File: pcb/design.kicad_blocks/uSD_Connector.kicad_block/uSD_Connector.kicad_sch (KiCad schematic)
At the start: 10 parts, among them J3 0472192001

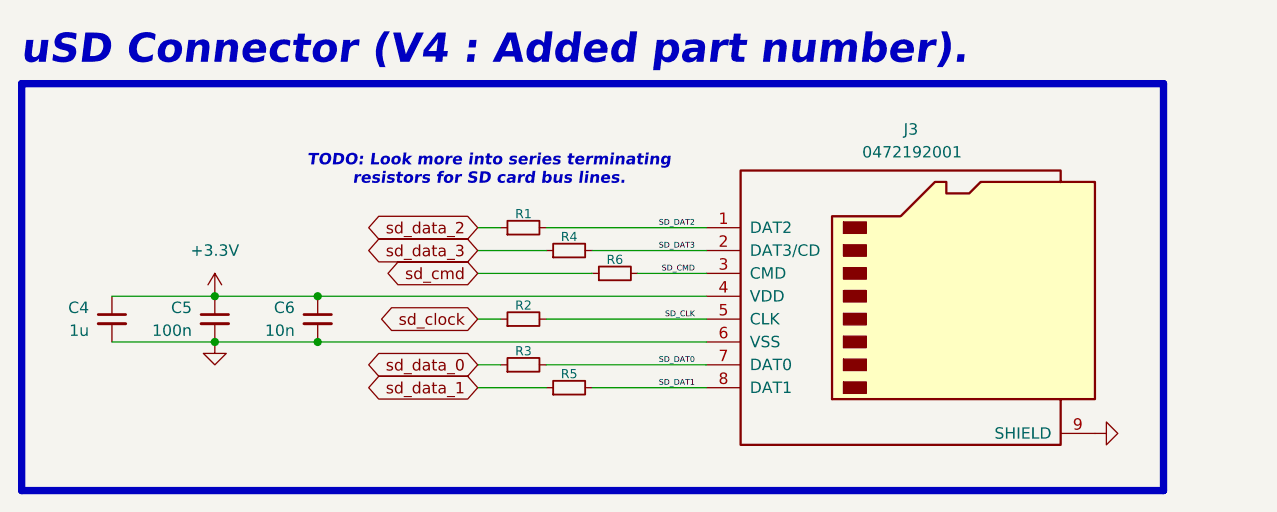
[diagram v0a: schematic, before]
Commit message: Addressed ERC issues.
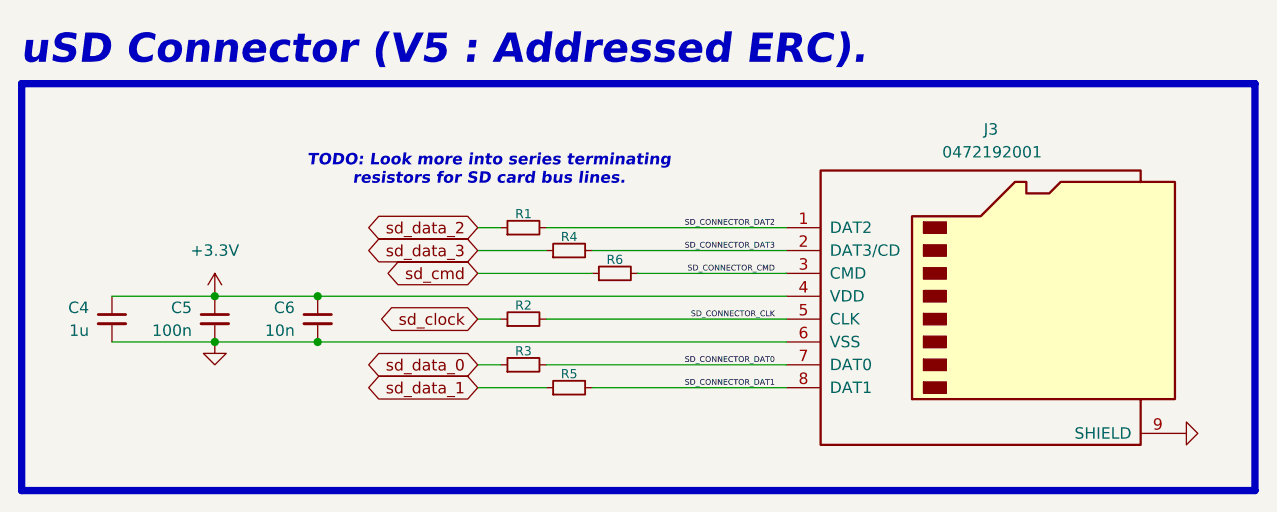
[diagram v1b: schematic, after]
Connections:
- net SD_CLK renamed SD_CONNECTOR_CLK
- net SD_CMD renamed SD_CONNECTOR_CMD
- net SD_DAT0 renamed SD_CONNECTOR_DAT0
- net SD_DAT1 renamed SD_CONNECTOR_DAT1
- net SD_DAT2 renamed SD_CONNECTOR_DAT2
- net SD_DAT3 renamed SD_CONNECTOR_DAT3
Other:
- note added: "uSD Connector (V5 : Addressed ERC)."
- note removed: "uSD Connector (V4 : Added part number)."
- moved on the sheet: J3
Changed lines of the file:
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@@
 	(rectangle
 		(start 340.487 166.878)
-		(end 467.36 212.09)
+		(end 477.52 212.09)
 		(stroke
 			(width 0.8128)
@@
 		)
 	)
-	(text "uSD Connector (V4 : Added part number)."
+	(text "uSD Connector (V5 : Addressed ERC)."
 		(exclude_from_sim no)
 		(at 340.36 165.1 0)
@@
 	(wire
 		(pts
-			(xy 398.78 182.88) (xy 416.56 182.88)
-		)
-		(stroke
-			(width 0)
-			(type default)
-		)
-	)
-	(wire
-		(pts
-			(xy 403.86 200.66) (xy 416.56 200.66)
-		)
-		(stroke
-			(width 0)
-			(type default)
-		)
-	)
-	(wire
-		(pts
-			(xy 373.38 195.58) (xy 416.56 195.58)
-		)
-		(stroke
-			(width 0)
-			(type default)
-		)
-	)
-	(wire
-		(pts
 			(xy 361.95 195.58) (xy 350.52 195.58)
 		)
@@
 	(wire
 		(pts
-			(xy 403.86 185.42) (xy 416.56 185.42)
-		)
-		(stroke
-			(width 0)
-			(type default)
-		)
-	)
-	(wire
-		(pts
-			(xy 398.78 198.12) (xy 416.56 198.12)
+			(xy 373.38 190.5) (xy 425.45 190.5)
+		)
+		(stroke
+			(width 0)
+			(type default)
+		)
+	)
+	(wire
+		(pts
+			(xy 403.86 185.42) (xy 425.45 185.42)
 		)
 		(stroke
@@
 	(wire
 		(pts
+			(xy 408.94 187.96) (xy 425.45 187.96)
+		)
+		(stroke
+			(width 0)
+			(type default)
+		)
+	)
+	(wire
+		(pts
 			(xy 361.95 190.5) (xy 373.38 190.5)
 		)
@@
 	(wire
 		(pts
+			(xy 398.78 193.04) (xy 425.45 193.04)
+		)
+		(stroke
+			(width 0)
+			(type default)
+		)
+	)
+	(wire
+		(pts
+			(xy 403.86 200.66) (xy 425.45 200.66)
+		)
+		(stroke
+			(width 0)
+			(type default)
+		)
+	)
+	(wire
+		(pts
 			(xy 393.7 182.88) (xy 391.16 182.88)
 		)
@@
 	(wire
 		(pts
+			(xy 398.78 198.12) (xy 425.45 198.12)
+		)
+		(stroke
+			(width 0)
+			(type default)
+		)
+	)
+	(wire
+		(pts
+			(xy 373.38 195.58) (xy 425.45 195.58)
+		)
+		(stroke
+			(width 0)
+			(type default)
+		)
+	)
+	(wire
+		(pts
 			(xy 350.52 190.5) (xy 361.95 190.5)
 		)
@@
 	(wire
 		(pts
-			(xy 373.38 190.5) (xy 416.56 190.5)
-		)
-		(stroke
-			(width 0)
-			(type default)
-		)
-	)
-	(wire
-		(pts
-			(xy 398.78 193.04) (xy 416.56 193.04)
+			(xy 398.78 182.88) (xy 425.45 182.88)
 		)
 		(stroke
@@
 		)
 	)
-	(wire
-		(pts
-			(xy 408.94 187.96) (xy 416.56 187.96)
-		)
-		(stroke
-			(width 0)
-			(type default)
-		)
-	)
-	(label "SD_CMD"
-		(at 415.29 187.96 180)
+	(label "SD_CONNECTOR_CMD"
+		(at 424.18 187.96 180)
 		(effects
 			(font
@@
 		)
 	)
-	(label "SD_CLK"
-		(at 415.29 193.04 180)
+	(label "SD_CONNECTOR_CLK"
+		(at 424.18 193.04 180)
 		(effects
 			(font
@@
 		)
 	)
-	(label "SD_DAT0"
-		(at 415.29 198.12 180)
+	(label "SD_CONNECTOR_DAT0"
+		(at 424.18 198.12 180)
 		(effects
 			(font
@@
 		)
 	)
-	(label "SD_DAT3"
-		(at 415.29 185.42 180)
+	(label "SD_CONNECTOR_DAT3"
+		(at 424.18 185.42 180)
 		(effects
 			(font
@@
 		)
 	)
-	(label "SD_DAT2"
-		(at 415.29 182.88 180)
+	(label "SD_CONNECTOR_DAT2"
+		(at 424.18 182.88 180)
 		(effects
 			(font
@@
 		)
 	)
-	(label "SD_DAT1"
-		(at 415.29 200.66 180)
+	(label "SD_CONNECTOR_DAT1"
+		(at 424.18 200.66 180)
 		(effects
 			(font
@@
 	(symbol
 		(lib_id "Connector:Micro_SD_Card")
-		(at 439.42 190.5 0)
+		(at 448.31 190.5 0)
 		(unit 1)
 		(exclude_from_sim no)
@@
 		(dnp no)
 		(property "Reference" "J3"
-			(at 439.293 171.958 0)
+			(at 448.183 171.958 0)
 			(effects
 				(font
@@
 		)
 		(property "Value" "0472192001"
-			(at 439.42 174.498 0)
+			(at 448.31 174.498 0)
 			(effects
 				(font
@@
 		)
 		(property "Footprint" "pcb:microSD_HC_Molex_47219-2001"
-			(at 468.63 182.88 0)
+			(at 477.52 182.88 0)
 			(effects
 				(font
@@
 		)
 		(property "Datasheet" "https://www.we-online.com/components/products/datasheet/693072010801.pdf"
-			(at 439.42 190.5 0)
+			(at 448.31 190.5 0)
 			(effects
 				(font
@@
 		)
 		(property "Description" "Micro SD Card Socket"
-			(at 439.42 190.5 0)
+			(at 448.31 190.5 0)
 			(effects
 				(font
@@
 	(symbol
 		(lib_id "power:GND")
-		(at 459.74 205.74 90)
+		(at 468.63 205.74 90)
 		(unit 1)
 		(exclude_from_sim no)
@@
 		(fields_autoplaced yes)
 		(property "Reference" "#PWR026"
-			(at 466.09 205.74 0)
+			(at 474.98 205.74 0)
 			(effects
 				(font
@@
 		)
 		(property "Value" "GND"
-			(at 463.55 205.7399 90)
+			(at 472.44 205.7399 90)
 			(effects
 				(font
@@
 		)
 		(property "Footprint" ""
-			(at 459.74 205.74 0)
+			(at 468.63 205.74 0)
 			(effects
 				(font
@@
 		)
 		(property "Datasheet" ""
-			(at 459.74 205.74 0)
+			(at 468.63 205.74 0)
 			(effects
 				(font
@@
 		)
 		(property "Description" "Power symbol creates a global label with name \"GND\" , ground"
-			(at 459.74 205.74 0)
-			(effects
-				(font
+			(at 468.63 205.74 0)
+			(effects
+				(font
